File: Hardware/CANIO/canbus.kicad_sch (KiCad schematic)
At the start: 3 parts, among them J201 CAN, J202 CAN, U201 MCP25625-x-SS

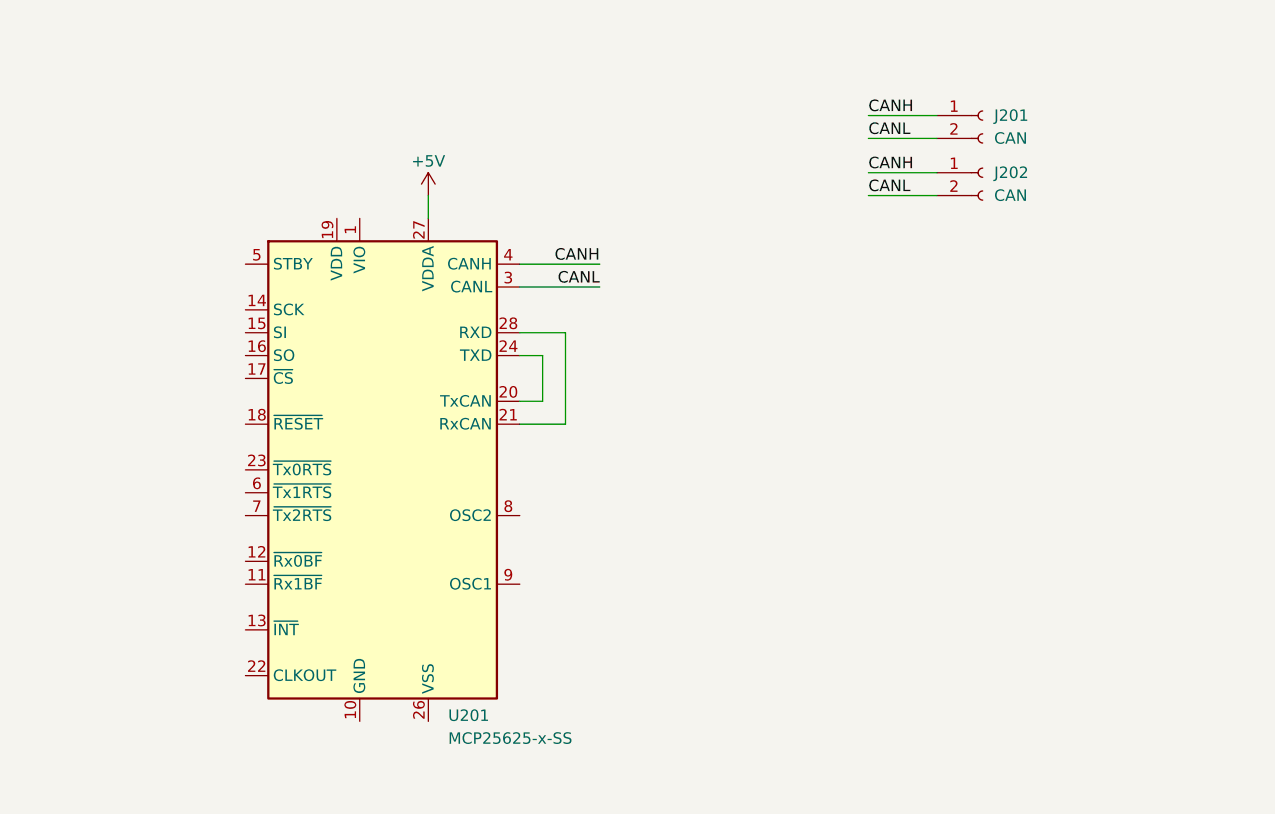
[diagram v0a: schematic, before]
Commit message: Add more boilerplate
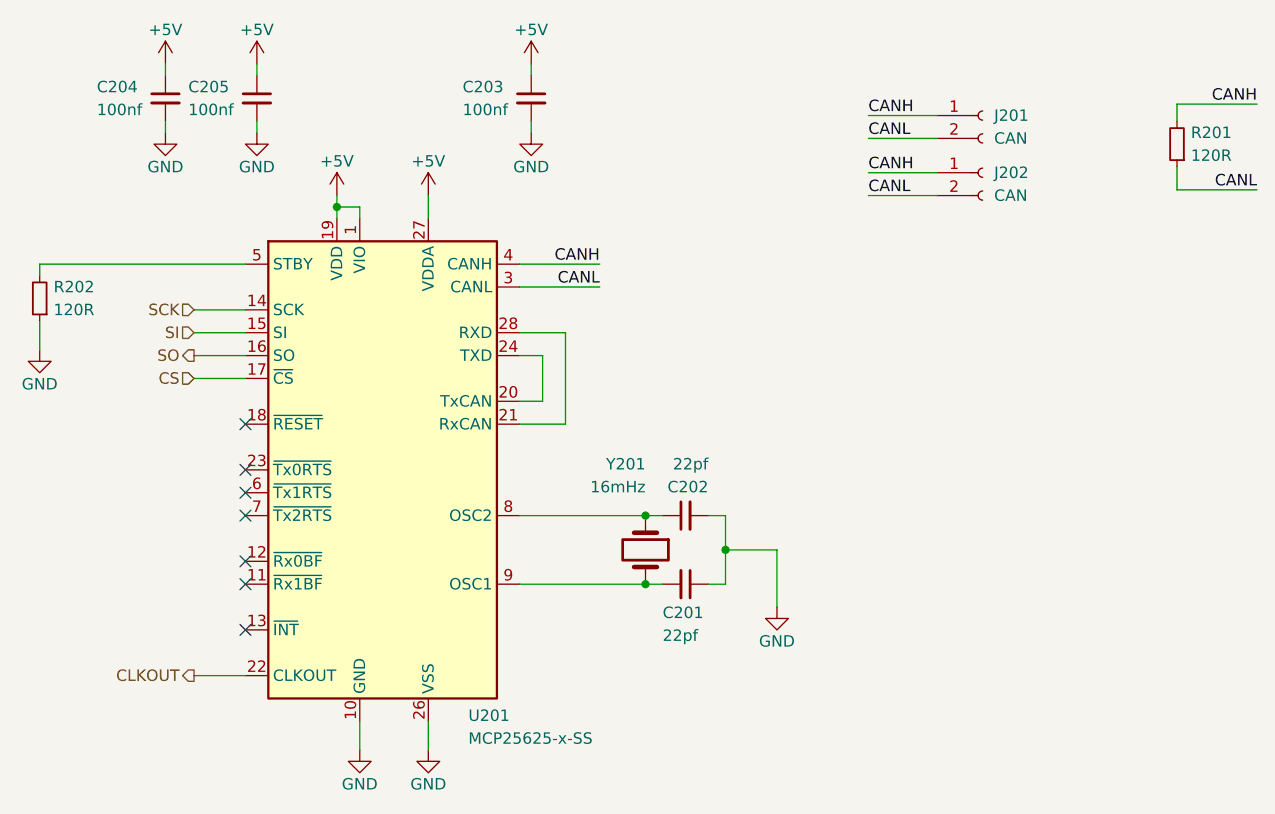
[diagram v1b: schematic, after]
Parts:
- added C201, C202: 22pf, Capacitor_SMD:C_0201_0603Metric, symbol Device:C_Small
- added C203, C204, C205: 100nf, Capacitor_SMD:C_0805_2012Metric, symbol Device:C_Small
- added R201: 120R, Resistor_THT:R_Axial_DIN0207_L6.3mm_D2.5mm_P10.16mm_Horizontal, symbol Device:R_Small
- added R202: 120R, Resistor_SMD:R_0805_2012Metric, symbol Device:R_Small
- added Y201: 16mHz, Crystal:Crystal_SMD_HC49-SD, symbol Device:Crystal
- J201, J202: footprint (none) -> Connector_Wire:SolderWire-0.5sqmm_1x02_P4.8mm_D0.9mm_OD2.3mm_Relief
- U201: LCSC# (none) -> C628816
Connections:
- net +5V: now also U201.1 (VIO), U201.19 (VDD), C203.1, C204.1, C205.1
- net CANH: now also R201.2
- net CANL: now also R201.1
- net GND: now reaches U201.10 (GND)
- net GND: now also U201.26 (VSS), C201.1, C202.2, C203.2, C204.2, C205.2, R202.1
- net SCK: now reaches U201.14 (SCK)
- net SI: now reaches U201.15 (SI)
- net SO: now reaches U201.16 (SO)
- net CS: now reaches U201.17 (~{CS})
- net CLKOUT: now reaches U201.22 (CLKOUT)
- net at U201.5 (STBY): now also R202.2
- net at U201.8 (OSC2): now also C202.1, Y201.1
- net at U201.9 (OSC1): now also C201.2, Y201.2
- no-connect marks 0 -> 7
